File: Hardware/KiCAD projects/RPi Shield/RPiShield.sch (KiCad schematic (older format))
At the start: 8 parts, among them J1 USB_OTG

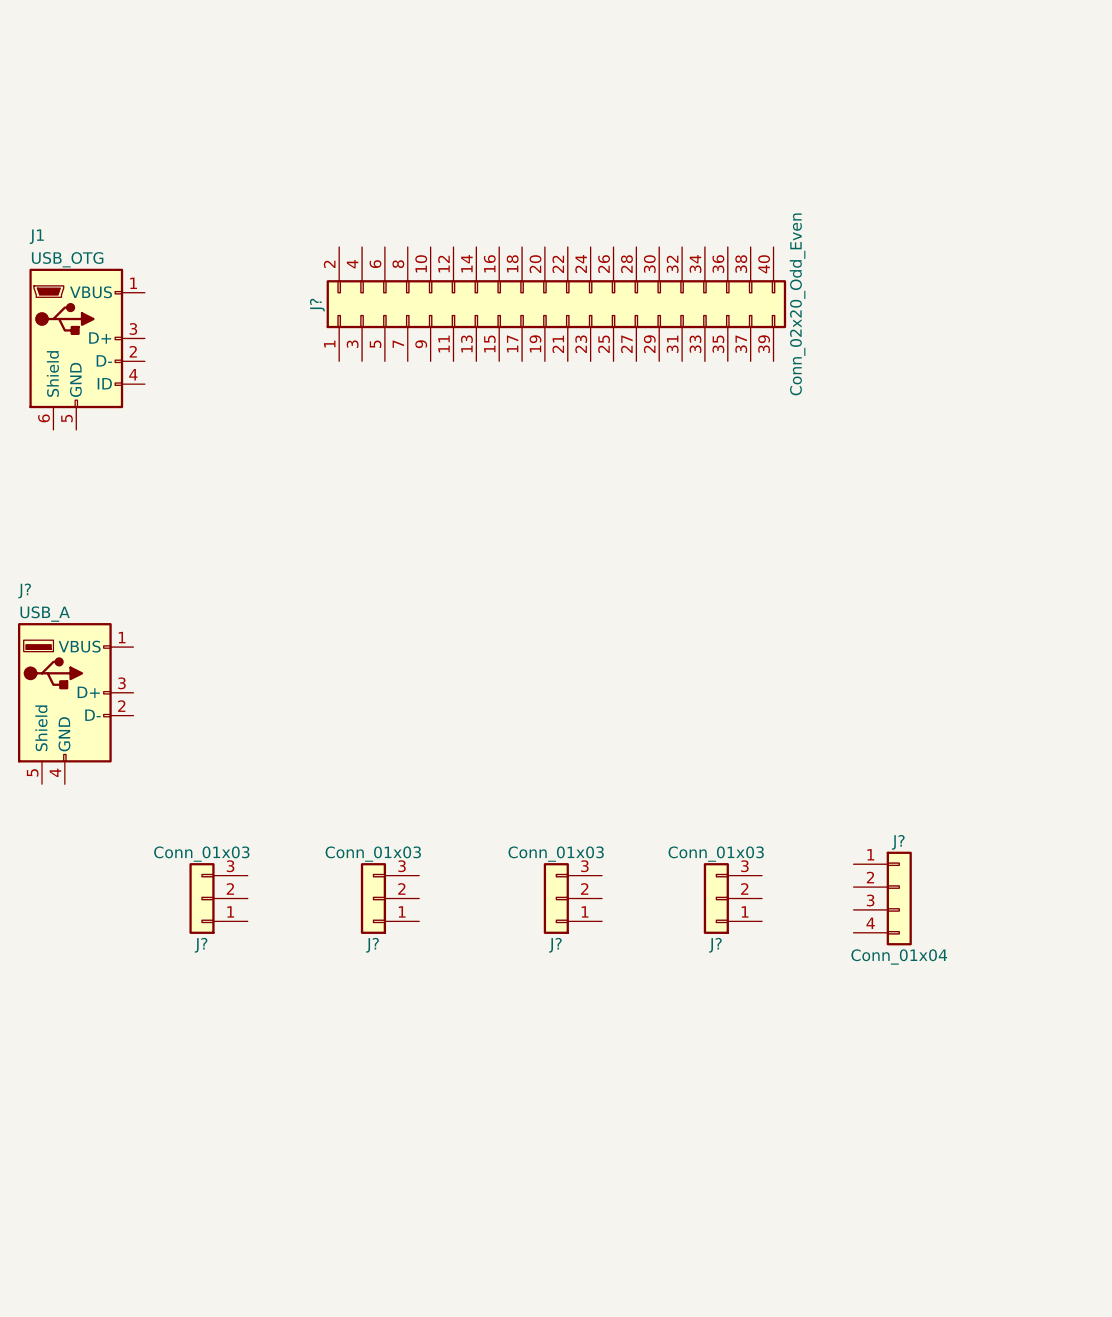
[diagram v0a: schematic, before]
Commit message: Robot PCB schematic work
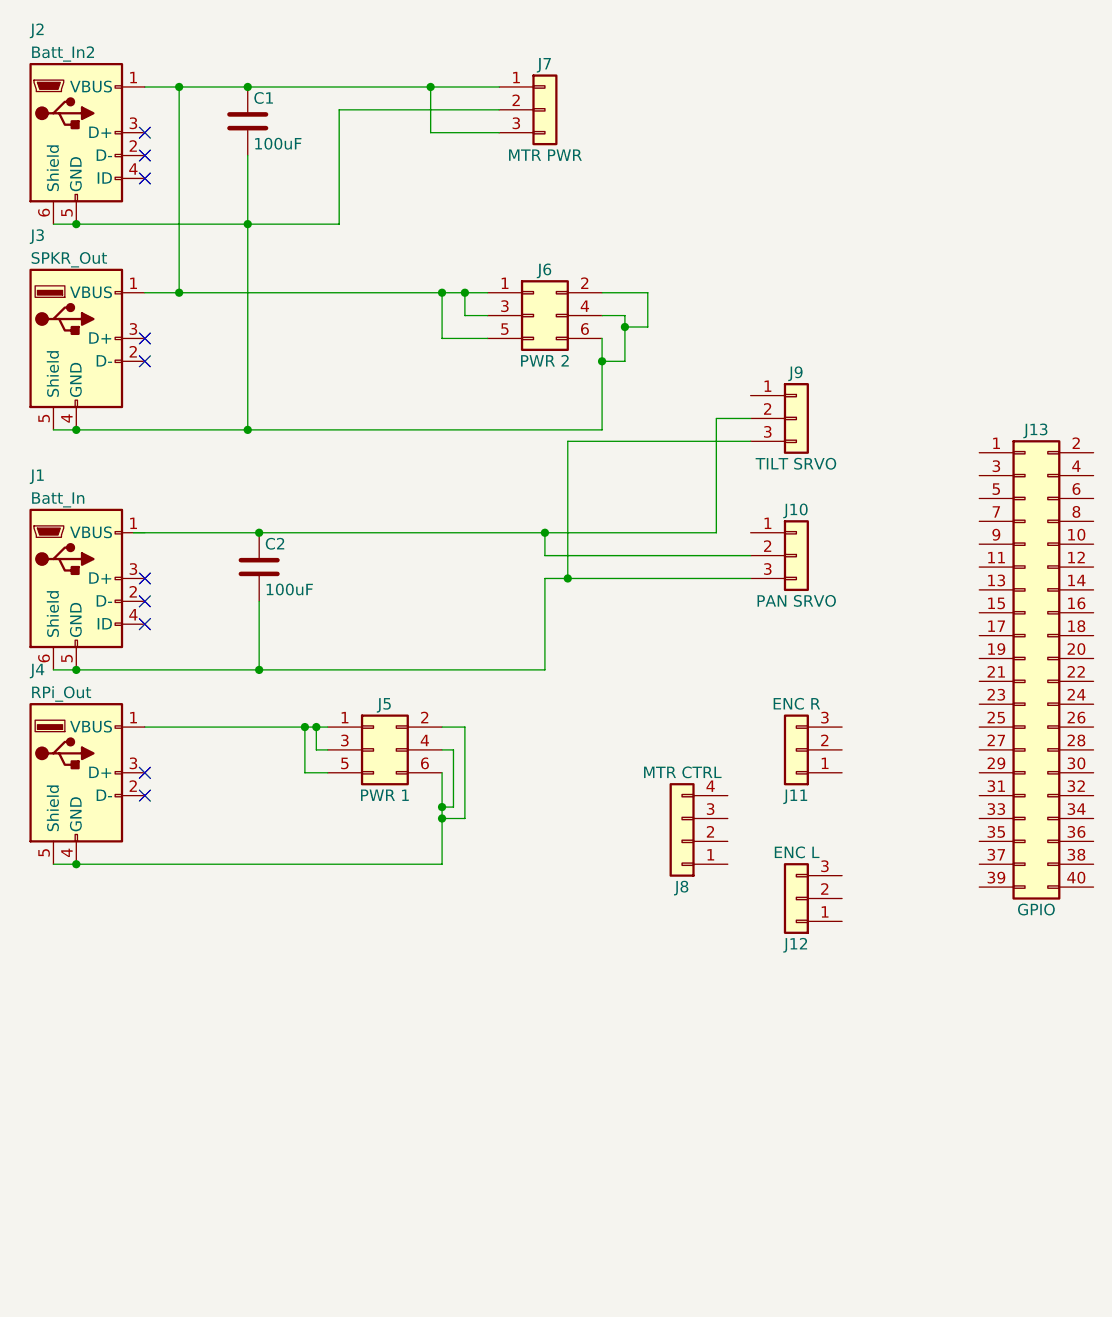
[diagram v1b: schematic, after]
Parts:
- added C1, C2: 100uF, symbol C
- added J2: Batt_In2, symbol USB_OTG
- added J4: RPi_Out, symbol USB_A
- added J5: PWR 1, symbol Conn_02x03_Odd_Even
- added J6: PWR 2, symbol Conn_02x03_Odd_Even
- added J7: MTR PWR, symbol Conn_01x03
- J1: value USB_OTG -> Batt_In
- J10: renamed from J?; value Conn_01x03 -> PAN SRVO
- J11: renamed from J?; value Conn_01x03 -> ENC R
- J12: renamed from J?; value Conn_01x03 -> ENC L
- J13: renamed from J?; value Conn_02x20_Odd_Even -> GPIO
- J3: renamed from J?; value USB_A -> SPKR_Out
- J8: renamed from J?; value Conn_01x04 -> MTR CTRL
- J9: renamed from J?; value Conn_01x03 -> TILT SRVO
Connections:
- net at J1.5 (GND): now also J1.6 (Shield), J10.3 (Pin_3), J9.3 (Pin_3), C2.2
- net at J3.1 (VBUS): now also C1.1, J2.1 (VBUS), J6.1 (Pin_1), J6.3 (Pin_3), J6.5 (Pin_5), J7.1 (Pin_1), J7.3 (Pin_3)
- net at J3.4 (GND): now also J3.5 (Shield), C1.2, J2.5 (GND), J2.6 (Shield), J6.2 (Pin_2), J6.4 (Pin_4), J6.6 (Pin_6), J7.2 (Pin_2)
- net at J9.2 (Pin_2): now also J10.2 (Pin_2), C2.1
- new net: J4.1 (VBUS), J5.1 (Pin_1), J5.3 (Pin_3), J5.5 (Pin_5)
- new net: J4.4 (GND), J4.5 (Shield), J5.2 (Pin_2), J5.4 (Pin_4), J5.6 (Pin_6)
- no-connect marks 0 -> 10
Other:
- moved on the sheet: J1, J10, J11, J12, J13, J3, J8, J9

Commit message: Kicad library stuff
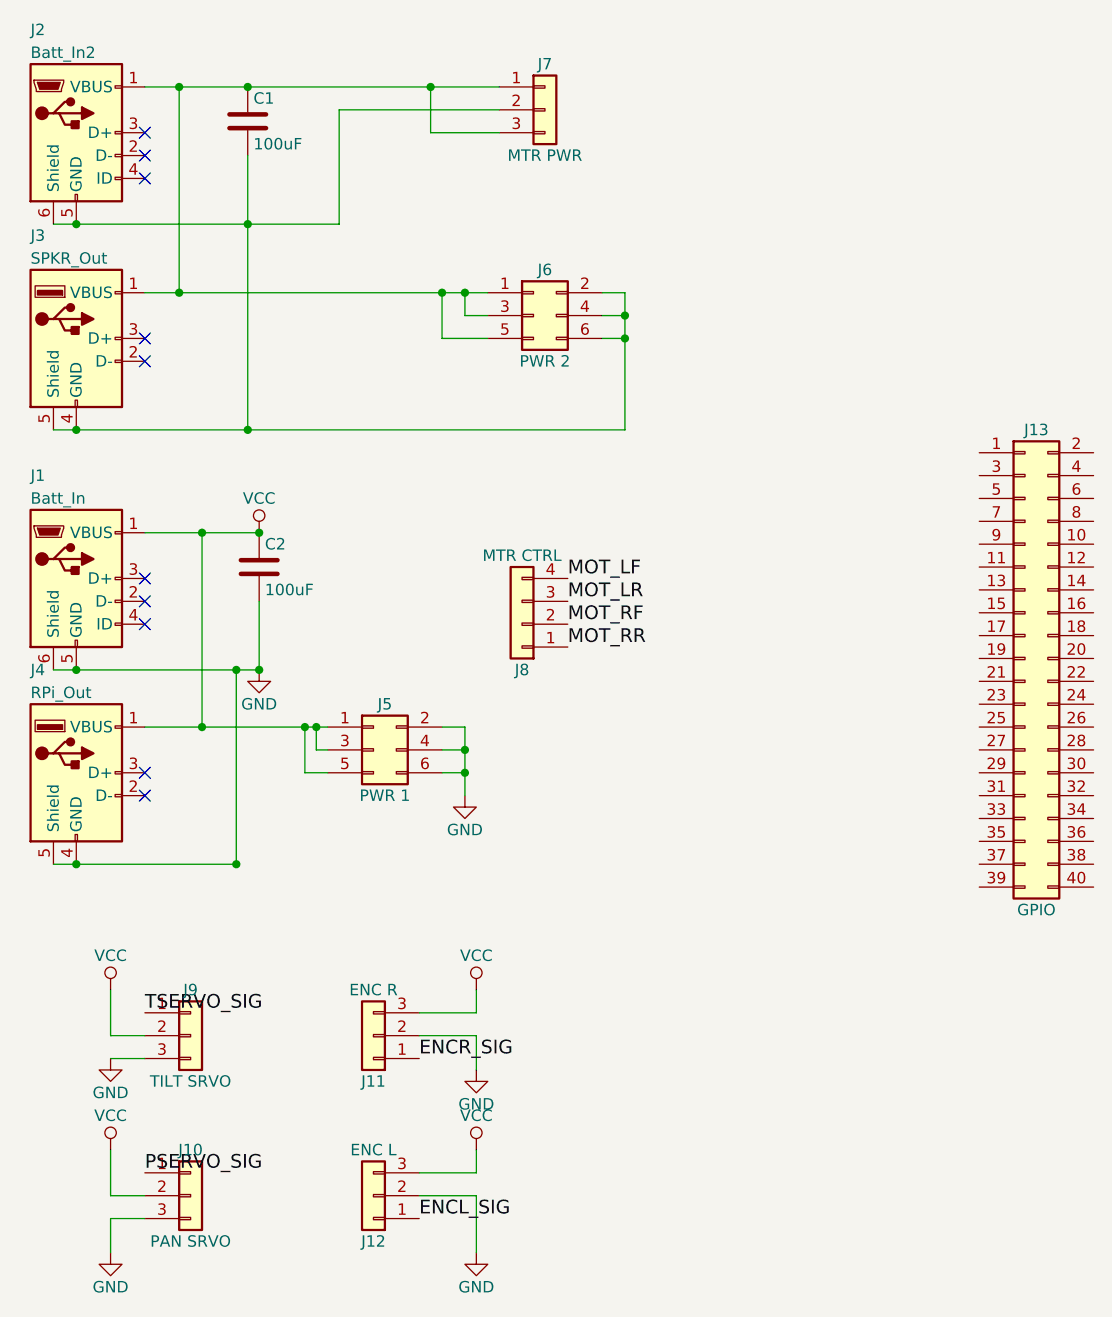
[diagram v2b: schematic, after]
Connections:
- net VCC: now reaches J1.1 (VBUS)
- net VCC: now also C2.1, J10.2 (Pin_2), J11.3 (Pin_3), J12.3 (Pin_3), J4.1 (VBUS), J5.1 (Pin_1), J5.3 (Pin_3), J5.5 (Pin_5), J9.2 (Pin_2)
- net GND: now reaches C2.2, J1.5 (GND), J1.6 (Shield), J10.3 (Pin_3), J9.3 (Pin_3)
- net GND: now also J11.2 (Pin_2), J12.2 (Pin_2), J4.4 (GND), J4.5 (Shield), J5.2 (Pin_2), J5.4 (Pin_4), J5.6 (Pin_6)
- net TSERVO_SIG: now reaches J9.1 (Pin_1)
- net PSERVO_SIG: now reaches J10.1 (Pin_1)
- net ENCR_SIG: now reaches J11.1 (Pin_1)
- net ENCL_SIG: now reaches J12.1 (Pin_1)
- net MOT_RR: now reaches J8.1 (Pin_1)
- net MOT_RF: now reaches J8.2 (Pin_2)
- net MOT_LR: now reaches J8.3 (Pin_3)
- net MOT_LF: now reaches J8.4 (Pin_4)
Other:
- moved on the sheet: J10, J11, J12, J8, J9
